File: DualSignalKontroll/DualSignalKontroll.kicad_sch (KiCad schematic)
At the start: 56 parts, among them J6 Signal A, J7 Signal B, J8 Screw_Terminal_01x04, Q1 BC547, Q2 BC547, Q3 BC547, Q4 BC547, Q5 BC547, Q6 BC547, SW1 Debug, U1 L7805, U2 PC817, U3 PC817, U4 PC817, U5 PC817, U6 PC817

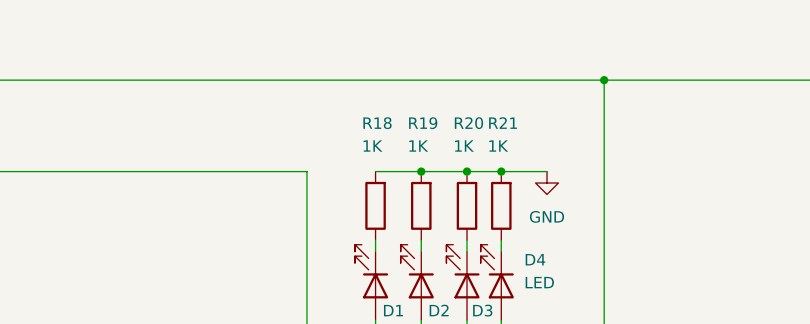
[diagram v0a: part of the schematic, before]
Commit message: updated schema
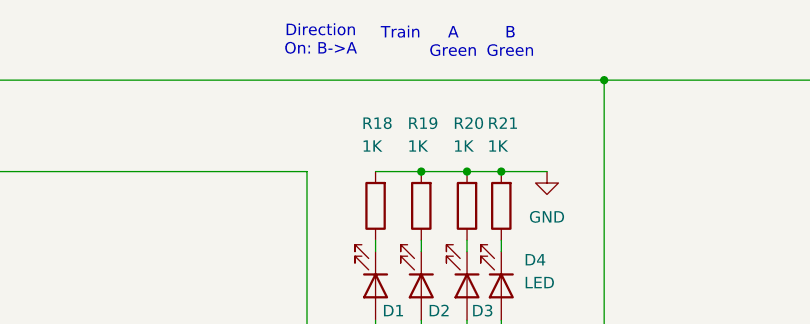
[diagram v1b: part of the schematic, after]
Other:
- note added: "A Green"
- note added: "B Green"
- note added: "Direction On: B->A"
- note added: "Train"
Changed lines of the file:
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@@
+		)
+	)
+	(text "A\nGreen"
+		(exclude_from_sim no)
+		(at 210.566 25.146 0)
+		(effects
+			(font
+				(size 1.27 1.27)
+			)
+		)
+	)
+	(text "Train"
+		(exclude_from_sim no)
+		(at 204.724 24.13 0)
+		(effects
+			(font
+				(size 1.27 1.27)
+			)
 		)
 	)
@@
 		)
 	)
+	(text "B\nGreen"
+		(exclude_from_sim no)
+		(at 216.916 25.146 0)
+		(effects
+			(font
+				(size 1.27 1.27)
+			)
+		)
+	)
 	(text "1.0"
 		(exclude_from_sim no)
@@
 		(effects
 			(font
+				(size 1.27 1.27)
+			)
+		)
+	)
+	(text "Direction\nOn: B->A"
+		(exclude_from_sim no)
+		(at 195.834 24.892 0)
+		(effects
+			(font
